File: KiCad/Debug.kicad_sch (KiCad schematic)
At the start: 0 parts

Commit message: he canviat el micro
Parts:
- added J3: Conn_01x03, symbol Connector_Generic:Conn_01x03
- added R16, R17: 100, symbol Device:R
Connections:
- new net: J3.1 (Pin_1), R16.2
- new net: J3.2 (Pin_2), R17.2
- new net GND: J3.3 (Pin_3)
- new net UART_RX: R17.1
- new net UART_TX: R16.1
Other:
- note added: "USART/DEBUG"

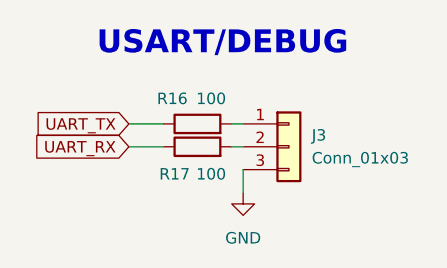
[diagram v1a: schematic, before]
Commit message: ERC i footprints
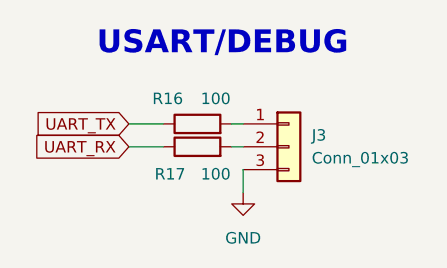
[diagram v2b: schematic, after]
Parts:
- J3: footprint (none) -> Connector_PinHeader_2.54mm:PinHeader_1x03_P2.54mm_Vertical
- R16, R17: footprint (none) -> Resistor_SMD:R_0805_2012Metric_Pad1.20x1.40mm_HandSolder
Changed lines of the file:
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@@
 		(dnp no)
 		(property "Reference" "R16"
-			(at 144.526 94.996 90)
+			(at 144.018 94.996 90)
 			(effects
 				(font
@@
 		)
 		(property "Value" "100"
-			(at 148.844 94.996 90)
-			(effects
-				(font
-					(size 1.27 1.27)
-				)
-			)
-		)
-		(property "Footprint" ""
+			(at 149.352 94.996 90)
+			(effects
+				(font
+					(size 1.27 1.27)
+				)
+			)
+		)
+		(property "Footprint" "Resistor_SMD:R_0805_2012Metric_Pad1.20x1.40mm_HandSolder"
 			(at 147.32 99.568 90)
 			(effects
@@
 		(dnp no)
 		(property "Reference" "R17"
-			(at 144.78 103.378 90)
+			(at 144.272 103.378 90)
 			(effects
 				(font
@@
 		)
 		(property "Value" "100"
-			(at 148.844 103.378 90)
-			(effects
-				(font
-					(size 1.27 1.27)
-				)
-			)
-		)
-		(property "Footprint" ""
+			(at 149.352 103.378 90)
+			(effects
+				(font
+					(size 1.27 1.27)
+				)
+			)
+		)
+		(property "Footprint" "Resistor_SMD:R_0805_2012Metric_Pad1.20x1.40mm_HandSolder"
 			(at 147.32 102.108 90)
 			(effects
@@
 			)
 		)
-		(property "Footprint" ""
+		(property "Footprint" "Connector_PinHeader_2.54mm:PinHeader_1x03_P2.54mm_Vertical"
 			(at 157.48 100.33 0)
 			(effects
